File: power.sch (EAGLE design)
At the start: 66 parts, among them CN1 21700, CN2 21700, CN3 21700, CN5 15PIN 0.5MM, Q1 SIRA36DP-T1-GE3, Q10 BSS123, Q2 SIRA36DP-T1-GE3, Q3 BSS123, Q4 BSS123, Q5 BSS123, Q6 BSS123, Q7 BSS123, Q8 BSS123, Q9 BSS123, U1 MAX17320G20+, U2 TCA6408AQPWRQ1, U3 TPS70918

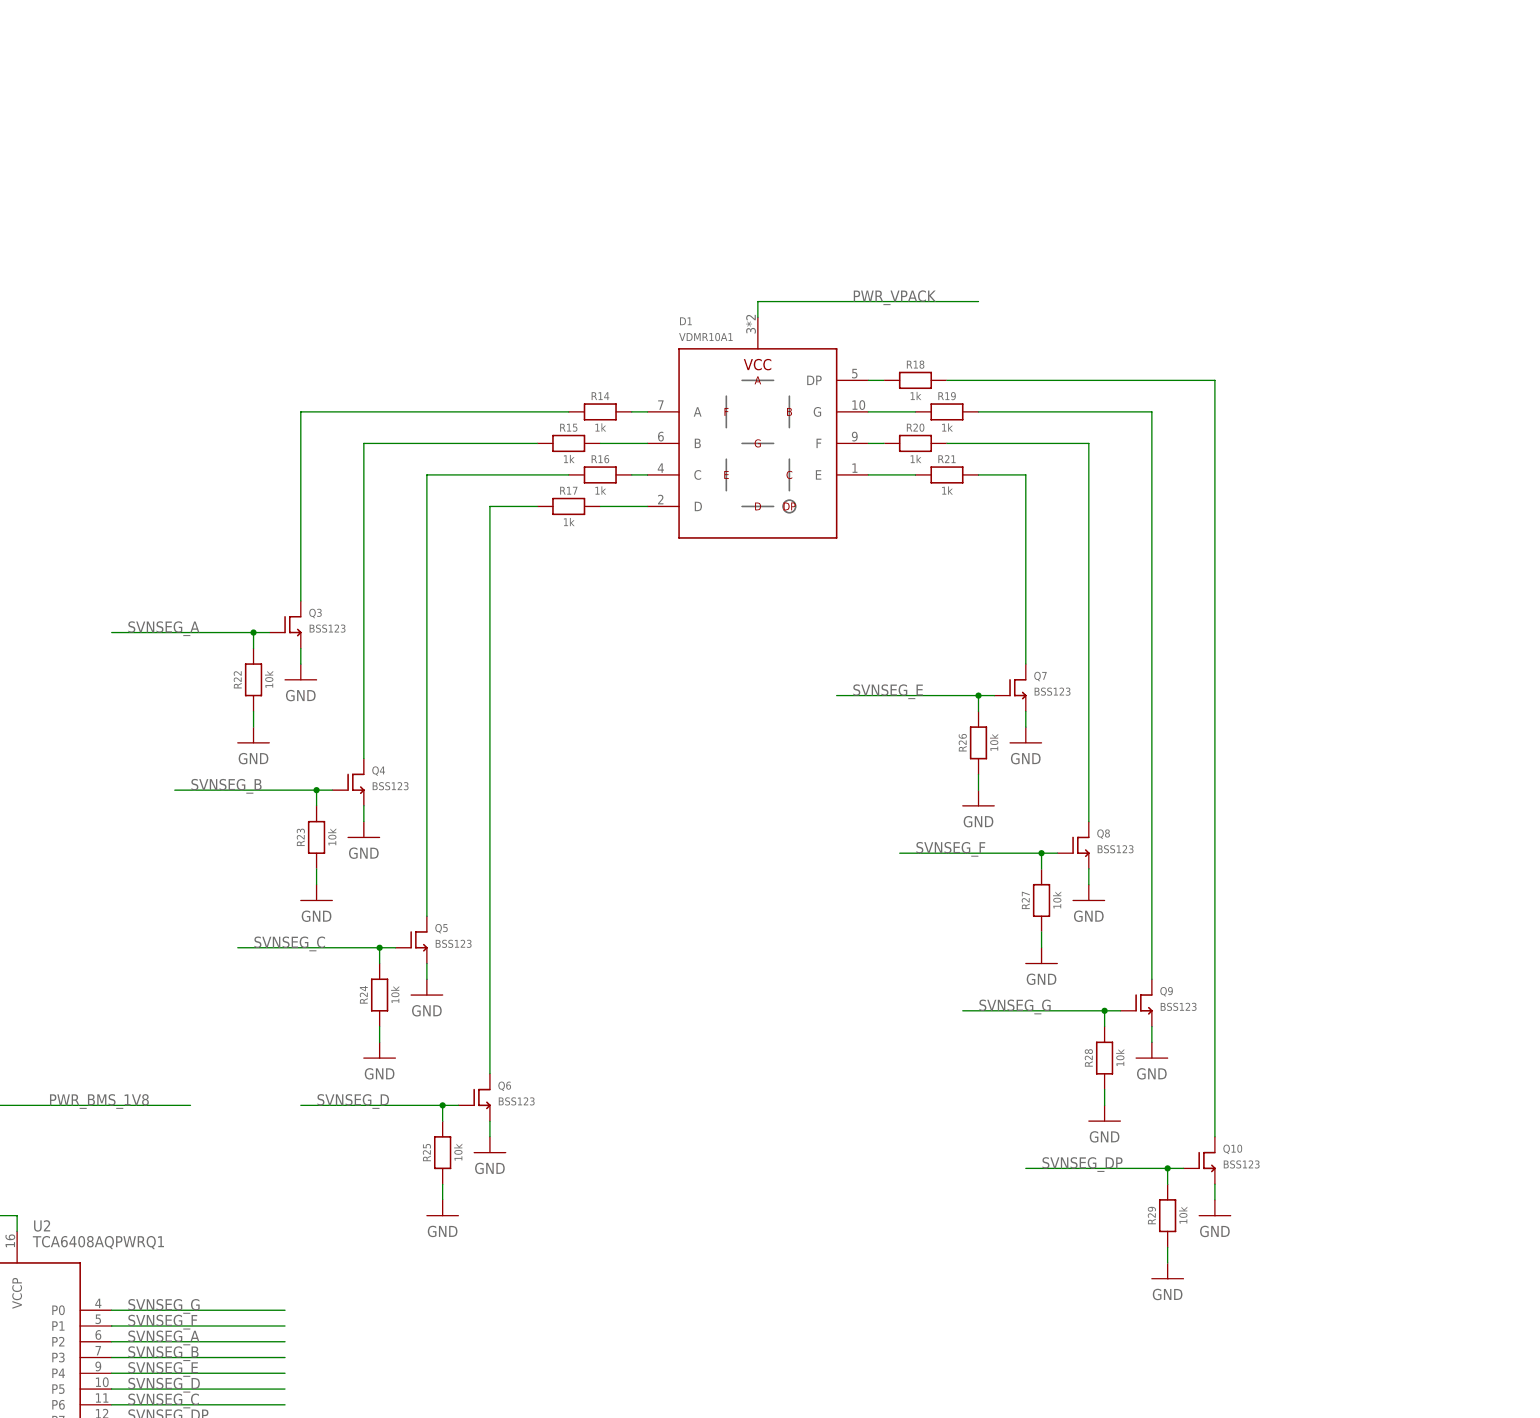
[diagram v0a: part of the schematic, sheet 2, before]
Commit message: Added I2C test points
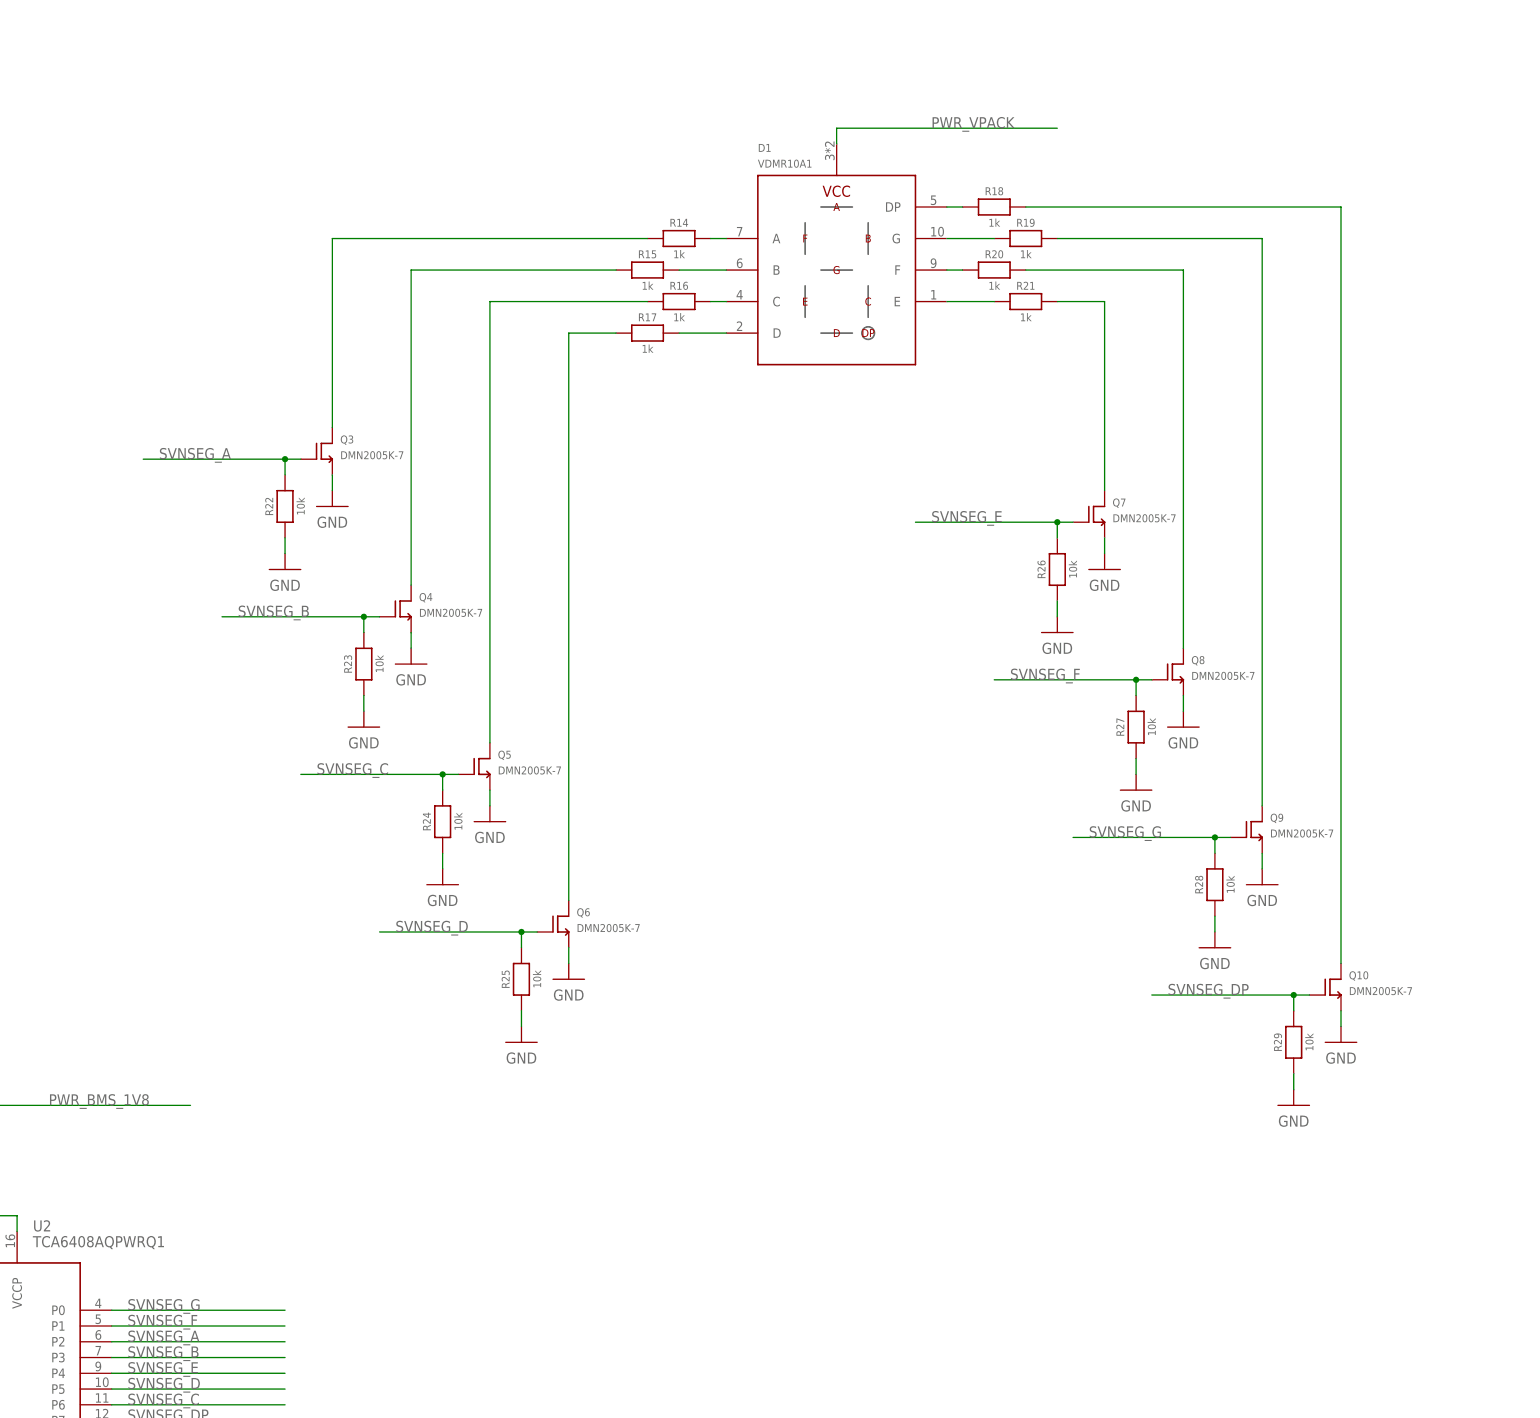
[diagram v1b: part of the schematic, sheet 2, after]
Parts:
- Q10, Q3, Q4, Q5, Q6, Q7, Q8, Q9: value BSS123 -> DMN2005K-7; device TRANSISTORs:BSS123 -> TRANSISTORs:DMN2005K-7
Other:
- moved on the sheet: D1, Q10, Q3, Q4, Q5, Q6, Q7, Q8, Q9, R14, R15, R16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

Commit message: started on power pcb
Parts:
- removed CN1, CN2: 21700, CONNECTORs:KEYSTONE1122
- removed D1: VDMR10A1, OPTO:VDMR10A1
- removed Q10, Q3, Q4, Q5, Q6, Q7, Q8, Q9: DMN2005K-7, TRANSISTORs:DMN2005K-7
- removed R19: 1k, r_0402:RC0402FR-071KL
- removed R22, R24, R26, R27, R28, R29, R30, R31: 10k, r_0402:RC0402FR-1010KL
- removed TP1, TP2, TP3, TP4: TEST_POINT_SQUARE, MISC:TEST_POINT_SQUARE
- added C14, C18, C19, C22, C24, C25, C26: 22uF 50V, CAPACITORS:GRM55DR72E105KW01L
- added C15, C16: 47pF 25V, c_0402:04023A470FAT2A
- added C17, C23, C27: 10uF 50V, CAPACITORS:C3225X7S1H106M250AB
- added C20: 0.1uF 50V, c_0603:06035L104K4T2A
- added C21: 100nF 16V, CAPACITORS:CL10B104KO8WPNC
- added CN10, CN11, CN12, CN15, CN16, CN17, CN18, CN21, CN22, CN23, CN24, CN4, CN6, CN9: 21700 CLIP, CONNECTORs:KEYSTONE247
- added MECH10, MECH2, MECH3, MECH4, MECH6, MECH8: 6mm x 3mm, MISC:MOUNTHOLE
- added U5: NCS20071, ICs:NCS20071SN2T1G
- added U6: LTM8055, ICs:LTM8055
- C11, C3: value 0.1uF 16V -> 47pF 25V; device c_0402:0402YD104KAT2A -> c_0402:04023A470FAT2A
- C12: value 2.2uF 6.3V -> 10uF 50V; device c_0603:06036D225KAT2A -> CAPACITORS:C3225X7S1H106M250AB
- C13: value 1uF 25V -> 22uF 50V; device c_0603:06033C105KAT2A -> CAPACITORS:GRM55DR72E105KW01L
- CN3: value 21700 -> 21700 CLIP; device CONNECTORs:KEYSTONE1122 -> CONNECTORs:KEYSTONE247
- CN5: value 15PIN 0.5MM -> 21700 CLIP; device CONNECTORs:SFV15R-1STE1HLF -> CONNECTORs:KEYSTONE247
- R13: value 10R -> 0R082; device r_0603:ERJ3EKF10R0V -> RESISTORS:RL73H3AR10FTDF
- R14: value 1k -> 150k; device r_0402:RC0402FR-071KL -> r_0402:RC0402FR-07150KL
- R15: value 1k -> 12k; device r_0402:RC0402FR-071KL -> r_0402:RC0402FR-0712KL
- R16, R18: value 1k -> 10k; device r_0402:RC0402FR-071KL -> r_0402:RC0402FR-1310KL
- R17: value 1k -> 45.3k; device r_0402:RC0402FR-071KL -> r_0402:RC0402FR-0745K3L
- R20: value 1k -> 75k; device r_0402:RC0402FR-071KL -> r_0402:RC0402FR-0775KL
- R21: value 1k -> 5.1k; device r_0402:RC0402FR-071KL -> r_0402:RC0402FR-135K1L
- R23: value 10k -> 45.3k; device r_0402:RC0402FR-1010KL -> r_0402:RC0402FR-0745K3L
- R25: device r_0402:RC0402FR-1010KL -> r_0402:RC0402FR-1310KL
- U2: value TCA6408AQPWRQ1 -> LTM8055; device ICs:TCA6408AQ -> ICs:LTM8055
- U3: value TPS70918 -> STM32G030C8; device ICs:TPS70918DBVT -> ICs:STM32G030C8T6
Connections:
- removed net N$13: D1.E, R21.1
- removed net N$19: Q4.D, R15.1
- removed net N$20: Q5.D, R16.1
- removed net N$21: Q6.D, R17.1
- removed net N$26: Q7.D, R21.2
- removed net N$29: Q10.D, R18.2
- removed net N$42: CN3.V+, Q1.S, R1.1, R2.1
- removed net N$44: R30.1, U2.!INT
- removed net N$50: R31.1, U2.!RESET
- removed net N$6: R13.2, U1.CSP
- removed net N$8: D1.C, R16.2
- removed net N$9: D1.D, R17.2
- removed net PACK_MID: CN1.V+, CN2.V-, R4.1, R5.1
- removed net PWR_BMS_1V8: C11.2, C12.2, C3.2, R30.2, R31.2, TP1.P$1, U2.VCCI, U2.VCCP, U3.VOUT
- removed net PWR_VPACK: C13.2, CN5.12, CN5.13, CN5.14, CN5.15, D1.VCC, Q2.S, R10.2, R12.2, U3.EN, U3.VIN
- removed net SVNSEG_A: Q3.G, R22.2, U2.P2
- removed net SVNSEG_B: Q4.G, R23.2, U2.P3
- removed net SVNSEG_C: Q5.G, R24.2, U2.P6
- removed net SVNSEG_D: Q6.G, R25.2, U2.P5
- removed net SVNSEG_DP: Q10.G, R29.2, U2.P7
- removed net SVNSEG_E: Q7.G, R26.2, U2.P4
- removed net SVNSEG_F: Q8.G, R27.2, U2.P1
- removed net SVNSEG_G: Q9.G, R28.2, U2.P0
- new net CHRG_ENABLE: R25.1, U2.RUN
- new net CHRG_IOUT_CTL: R18.1, U5.+
- new net N$17: U2.LL, U2.MODE
- new net N$22: CN11.1, CN4.1, CN6.1, CN9.1, R4.1
- new net N$23: R20.1, R21.1, U6.FB
- new net N$25: CN10.1, CN12.1, CN15.1, CN17.1, R5.1
- new net N$32: CN16.1, CN18.1, CN21.1, CN23.1, R3.1
- new net N$35: U6.LL, U6.MODE
- new net N$36: C16.2, U6.SS
- new net N$63: C2.1, C21.2, R5.2, U1.CELL2
- new net PWR_BAT_VPACK: C17.2, C27.2, Q2.S, R10.2, R12.2, R13.2, U2.I_OUT, U6.I_IN, U6.SV_IN, U6.V_IN
- new net PWR_SYS_19V: C18.2, C19.2, C22.2, C24.2, R20.2, U6.I_OUT, U6.V_OUT
- new net PWR_SYS_19V_EN: R16.1, U6.RUN
- new net PWR_SYS_VIN_COND: C12.2, C20.2, C23.2, U2.I_IN, U2.SV_IN, U2.V_IN, U5.V+
- net BMS_I2C_SCL: no longer CN5.11, TP2.P$1, U2.SCL
- net BMS_I2C_SDA: no longer CN5.10, TP3.P$1, U2.SDA
- net BMS_NALERT: no longer CN5.9
- net GND: now also C14.1, C15.1, C16.1, C17.1, C18.1, C19.1, C20.1, C22.1, C23.1, C24.1, C25.1, C26.1, C27.1, R15.2, R16.2, R17.1, R18.2, R21.2, R25.2, U2.SYNC, U5.V-, U6.GND, U6.SYNC; no longer CN5.1, CN5.2, CN5.3, CN5.4, CN5.5, CN5.6, Q10.S, Q3.S, Q4.S, Q5.S, Q6.S, Q7.S, Q8.S, Q9.S, R22.1, R24.1, R25.1, R26.1, R27.1, R28.1, R29.1, TP4.P$1, U2.ADDR, U3.GND
- net N$10: now also R17.2, U2.RT; no longer D1.DP, R18.1
- net N$11: now also C3.2, U2.COMP; no longer D1.G, R19.1
- net N$12: now also U2.CTL, U5.-, U5.OUT; no longer D1.F, R20.1
- net N$18: now also C11.2, U2.SS; no longer Q3.D, R14.1
- net N$27: now also R23.2, U6.RT; no longer Q8.D, R20.2
- net N$28: now also C15.2, U6.COMP; no longer Q9.D, R19.2
- net N$3: now also C21.1; no longer C2.1, R5.2, U1.CELL2
- net N$4: now also C13.2, C14.2, C25.2, C26.2, R13.1, R14.2, U2.V_OUT; no longer CN2.V+, CN3.V-, R3.1
- net N$5: now also CN22.1, CN24.1, Q1.S, R1.1, R2.1; no longer D1.A, R14.2
- net N$7: now also R14.1, R15.1, U2.FB; no longer D1.B, R15.2
- net PGND: now also CN3.1, CN5.1, U1.CSP; no longer CN1.V-, R13.1
